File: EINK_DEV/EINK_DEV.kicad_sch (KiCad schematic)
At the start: 77 parts, among them J1 FPC, J2 USB_B_Micro, J3 Conn_01x02, J4 Conn_01x03, J5 Conn_ARM_SWD_TagConnect_TC2030, J6 UART, J7 Conn_Coaxial, J8 GPIO_Header_Dev, Q1 NMOS, SW1 SW_Push, U1 STM32WB55CEUx, U2 TP4056-42-ESOP8, U3 DW01A, U5 AMS1117-3.3, Y1 32kHz768, Y2 32Mhz

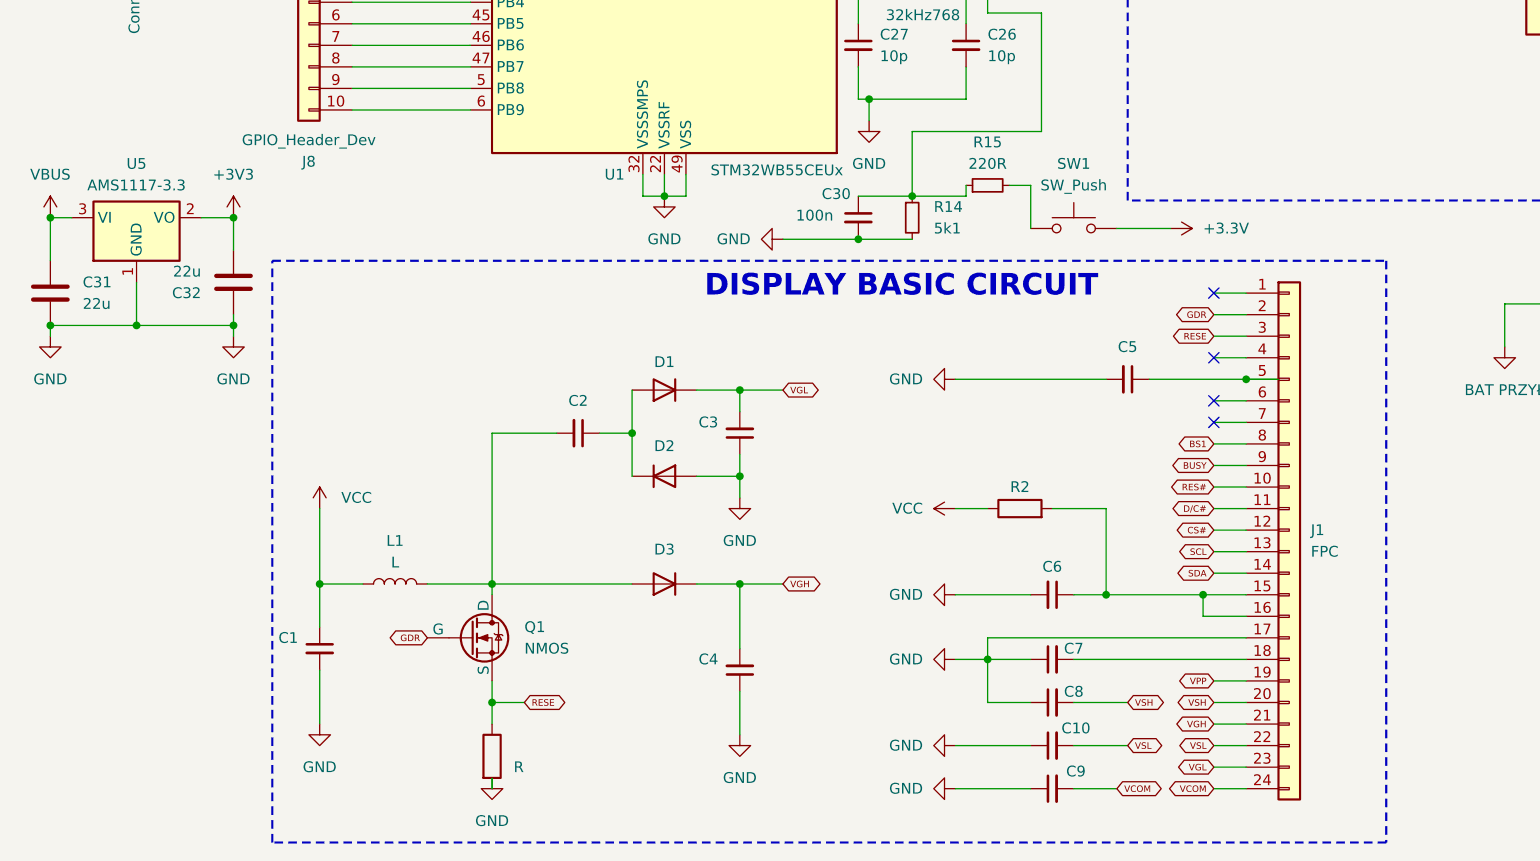
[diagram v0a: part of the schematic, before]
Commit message: Commit
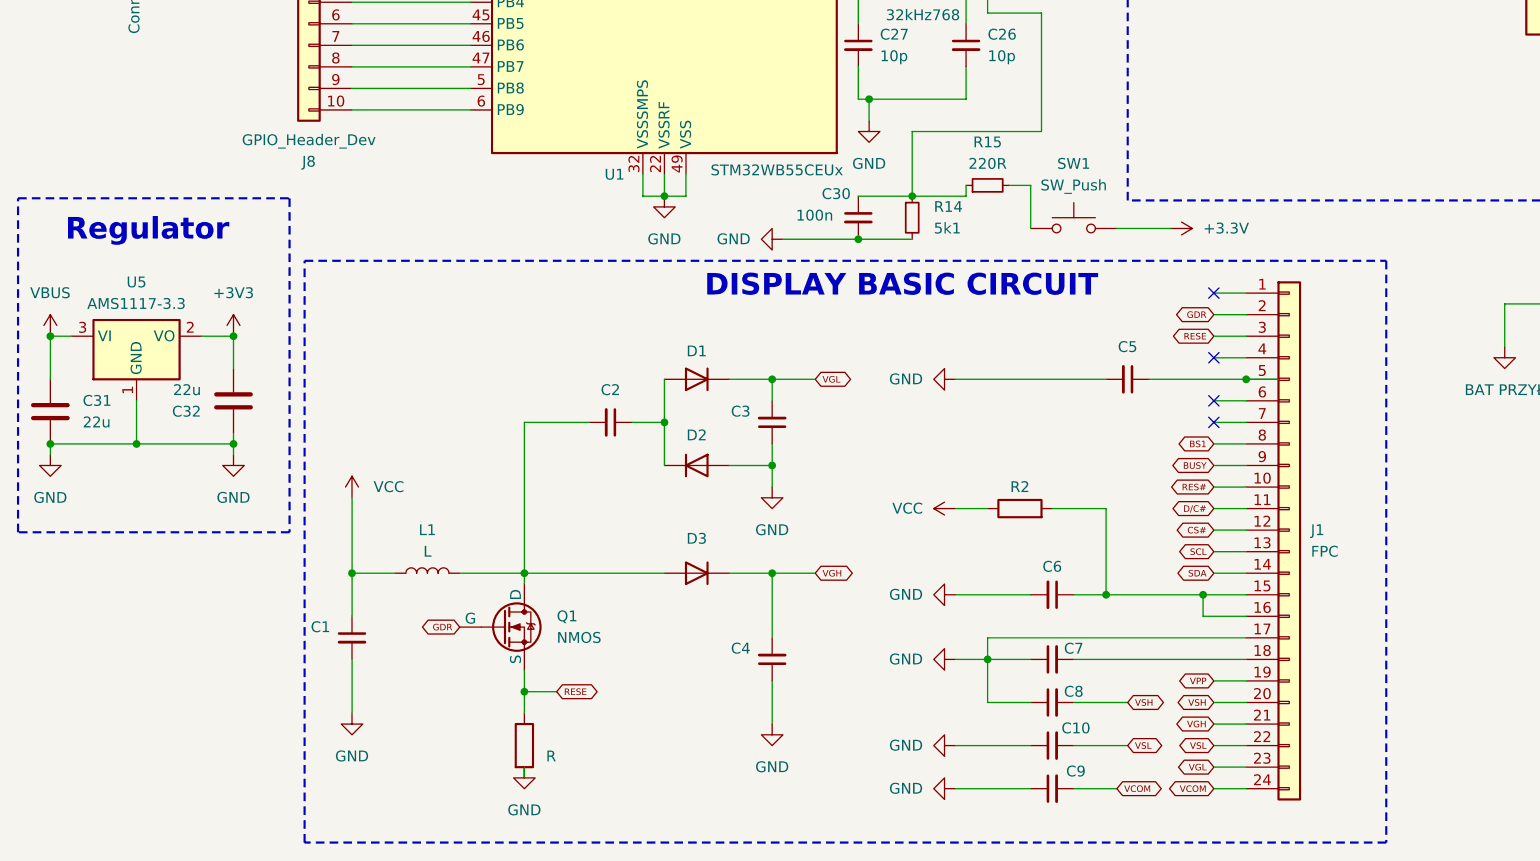
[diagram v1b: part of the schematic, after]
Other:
- note added: "Regulator"
- moved on the sheet: C1, C2, C3, C31, C32, C4, D1, D2, D3, L1, Q1, U5
